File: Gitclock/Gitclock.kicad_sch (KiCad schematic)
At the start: 4 parts

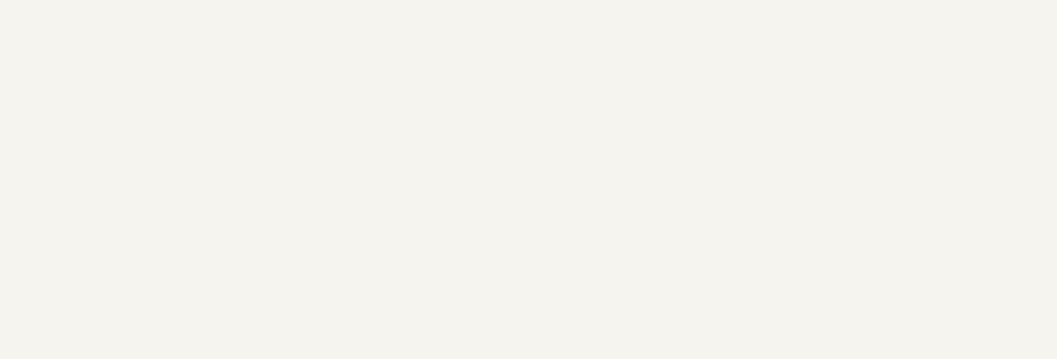
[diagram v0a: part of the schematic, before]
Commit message: Gitclock
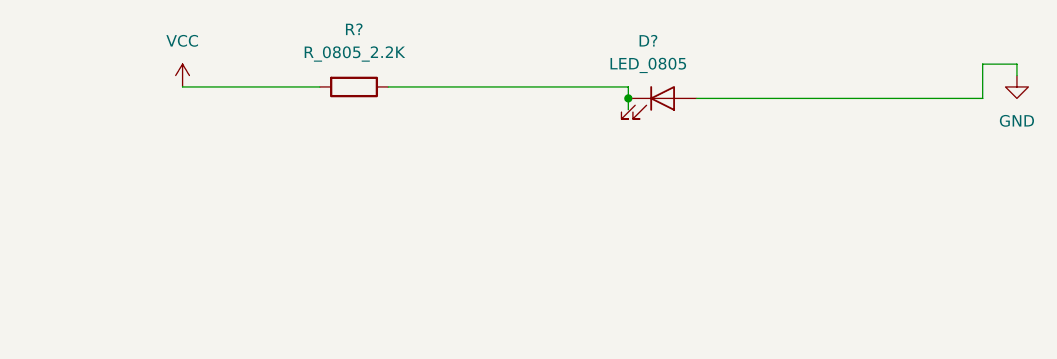
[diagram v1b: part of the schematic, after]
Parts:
- added D?: LED_0805, footprints:LED_0805_2012Metric, symbol HPS:LED_0805
- added R?: R_0805_2.2K, footprints:R_0805_2012Metric, symbol HPS:R_0805_2.2K
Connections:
- new net: D?.1 (K), R?.1
- new net GND: D?.2 (A)
- new net VCC: R?.2
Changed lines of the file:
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@@
 (kicad_sch (version 20211123) (generator eeschema)
   (paper "A4")
+  (junction (at 102.87 91.44) (diameter 0) (color 0 0 0 0)
+  )
+  (wire (pts (xy 142.24 91.44) (xy 142.24 87.63))
+    (stroke (width 0) (type default) (color 0 0 0 0))
+  )
+  (wire (pts (xy 146.05 87.63) (xy 146.05 88.9))
+    (stroke (width 0) (type default) (color 0 0 0 0))
+  )
+  (wire (pts (xy 102.87 91.44) (xy 102.87 92.71))
+    (stroke (width 0) (type default) (color 0 0 0 0))
+  )
+  (wire (pts (xy 110.49 91.44) (xy 142.24 91.44))
+    (stroke (width 0) (type default) (color 0 0 0 0))
+  )
+  (wire (pts (xy 76.2 90.17) (xy 102.87 90.17))
+    (stroke (width 0) (type default) (color 0 0 0 0))
+  )
+  (wire (pts (xy 142.24 87.63) (xy 146.05 87.63))
+    (stroke (width 0) (type default) (color 0 0 0 0))
+  )
+  (wire (pts (xy 102.87 90.17) (xy 102.87 91.44))
+    (stroke (width 0) (type default) (color 0 0 0 0))
+  )
+  (wire (pts (xy 53.34 90.17) (xy 68.58 90.17))
+    (stroke (width 0) (type default) (color 0 0 0 0))
+  )
   (symbol (lib_id "HPS:MountingHole") (at 45.72 179.07 0) (unit 1)
     (in_bom yes) (on_board yes) (fields_autoplaced)
@@
     )
   )
+  (symbol (lib_id "HPS:VCC") (at 53.34 90.17 0) (unit 1)
+    (in_bom yes) (on_board yes) (fields_autoplaced)
+    (property "Reference" "#PWR?" (id 0) (at 53.34 93.98 0)
+      (effects (font (size 1.27 1.27)) hide)
+    )
+    (property "Value" "VCC" (id 1) (at 53.34 85.09 0))
+    (property "Footprint" "" (id 2) (at 53.34 90.17 0)
+      (effects (font (size 1.27 1.27)) hide)
+    )
+    (property "Datasheet" "" (id 3) (at 53.34 90.17 0)
+      (effects (font (size 1.27 1.27)) hide)
+    )
+    (pin "1")
+  )
   (symbol (lib_id "HPS:MountingHole") (at 25.4 179.07 0) (unit 1)
     (in_bom yes) (on_board yes) (fields_autoplaced)
@@
     )
   )
+  (symbol (lib_id "HPS:R_0805_2.2K") (at 72.39 90.17 270) (unit 1)
+    (in_bom yes) (on_board yes) (fields_autoplaced)
+    (property "Reference" "R?" (id 0) (at 72.39 83.82 90))
+    (property "Value" "R_0805_2.2K" (id 1) (at 72.39 86.36 90))
+    (property "Footprint" "footprints:R_0805_2012Metric" (id 2) (at 72.39 85.852 90)
+      (effects (font (size 1.27 1.27)) hide)
+    )
+    (property "Datasheet" "https://www.digikey.com/en/products/detail/yageo/RC0805FR-072K2L/727676" (id 3) (at 72.39 87.63 0)
+      (effects (font (size 1.27 1.27)) hide)
+    )
+    (property "MFG" "N/A" (id 4) (at 66.04 90.17 0)
+      (effects (font (size 1.27 1.27)) hide)
+    )
+    (property "MPN" "N/A" (id 5) (at 63.5 90.17 0)
+      (effects (font (size 1.27 1.27)) hide)
+    )
+    (property "Digikey PN" "311-2.20KCRCT-ND" (id 6) (at 58.42 90.17 0)
+      (effects (font (size 1.27 1.27)) hide)
+    )
+    (property "Mouser PN" "N/A" (id 7) (at 55.88 90.17 0)
+      (effects (font (size 1.27 1.27)) hide)
+    )
+    (property "Power" "N/A" (id 8) (at 53.34 90.17 0)
+      (effects (font (size 1.27 1.27)) hide)
+    )
+    (property "Tolerance" "N/A" (id 9) (at 53.34 90.17 0)
+      (effects (font (size 1.27 1.27)) hide)
+    )
+    (pin "1")
+    (pin "2")
+  )
+  (symbol (lib_id "HPS:LED_0805") (at 106.68 91.44 0) (unit 1)
+    (in_bom yes) (on_board yes) (fields_autoplaced)
+    (property "Reference" "D?" (id 0) (at 105.0798 85.09 0))
+    (property "Value" "LED_0805" (id 1) (at 105.0798 87.63 0))
+    (property "Footprint" "footprints:LED_0805_2012Metric" (id 2) (at 107.95 102.87 0)
+      (effects (font (size 1.27 1.27)) hide)
+    )
+    (property "Datasheet" "https://www.we-online.de/katalog/datasheet/150080RS75000.pdf" (id 3) (at 106.68 91.44 0)
+      (effects (font (size 1.27 1.27)) hide)
+    )
+    (property "MFG" "Würth Elektronik" (id 4) (at 106.68 97.79 0)
+      (effects (font (size 1.27 1.27)) hide)
+    )
+    (property "MPN" "150080RS75000" (id 5) (at 106.68 100.33 0)
+      (effects (font (size 1.27 1.27)) hide)
+    )
+    (property "Digikey PN" "732-4984-1-ND" (id 6) (at 106.68 105.41 0)
+      (effects (font (size 1.27 1.27)) hide)
+    )
+    (property "Mouser PN" "N/A" (id 7) (at 106.68 107.95 0)
+      (effects (font (size 1.27 1.27)) hide)
+    )
+    (pin "1")
+    (pin "2")
+  )
   (symbol (lib_id "HPS:MountingHole") (at 25.4 186.69 0) (unit 1)
     (in_bom yes) (on_board yes) (fields_autoplaced)
@@
       (effects (font (size 1.27 1.27)) hide)
     )
+  )
+  (symbol (lib_id "HPS:GND") (at 146.05 88.9 0) (unit 1)
+    (in_bom yes) (on_board yes) (fields_autoplaced)
+    (property "Reference" "#PWR?" (id 0) (at 146.05 95.25 0)
+      (effects (font (size 1.27 1.27)) hide)
+    )
+    (property "Value" "GND" (id 1) (at 146.05 93.98 0))
+    (property "Footprint" "" (id 2) (at 146.05 88.9 0)
+      (effects (font (size 1.27 1.27)) hide)
+    )
+    (property "Datasheet" "" (id 3) (at 146.05 88.9 0)
+      (effects (font (size 1.27 1.27)) hide)
+    )
+    (pin "1")
   )
   (symbol (lib_id "HPS:MountingHole") (at 45.72 186.69 0) (unit 1)
@@
   )
   (symbol_instances
+    (path "/2c2c9064-4278-4cae-8cef-5f06f9b0ef6b"
+      (reference "#PWR?") (unit 1) (value "VCC") (footprint "")
+    )
+    (path "/b76389d4-f0e4-4569-b356-6c22f544bace"
+      (reference "#PWR?") (unit 1) (value "GND") (footprint "")
+    )
+    (path "/5060fb64-c5fc-4992-9356-3e6ce085d1f6"
+      (reference "D?") (unit 1) (value "LED_0805") (footprint "footprints:LED_0805_2012Metric")
+    )
     (path "/3078fc62-fc65-44c3-8730-e98e32046f59"
       (reference "H1") (unit 1) (value "MountingHole") (footprint "footprints:MountingHole_3.2mm_M3")
@@
       (reference "H4") (unit 1) (value "MountingHole") (footprint "footprints:MountingHole_3.2mm_M3")
     )
-  )
+    (path "/4563f1f1-b61c-4fb3-8057-693c3438b45b"
+      (reference "R?") (unit 1) (value "R_0805_2.2K") (footprint "footprints:R_0805_2012Metric")
+    )
+  )
